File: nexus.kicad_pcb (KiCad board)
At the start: 2 copper layers, 101.5 x 126.2 mm, 112 parts, among them J1 PIN6-9_Breakout, J10 Screw_Terminal_01x02, J11 24V_Lockout_Key_Switch, J12 XT60-M, J13 PT_1, J14 PT_4, J15 PT_2, J16 PT_5, J17 PT_3, J18 PT_6, J19 4-Pin Load Cell, J2 PIN10-13_Breakout, J20 5-Pin Load Cell, J21 Ignitor Screw Terminal, J3 Valve_1_PWR, J4 Valve_4_PWR, J5 Valve_2_PWR, J6 Valve_5_PWR, J7 Valve_3_PWR, J8 Valve_6_PWR, J9 Screw_Terminal_01x04, K1 G5LE-1, K2 G5LE-1, Q1 BSS138, Q2 BSS138, Q3 BSS138, Q4 BSS138, Q5 BSS138, Q6 BSS138, Q7 BSS138, Q8 BSS138, U1 ESP32-S3, U2 ADS112C04, U3 ADS112C04, U4 ADS112C04, U5 ADS112C04, U6 XC6206P332MR, U7 TPS5430DDA, U8 TPS5430DDA

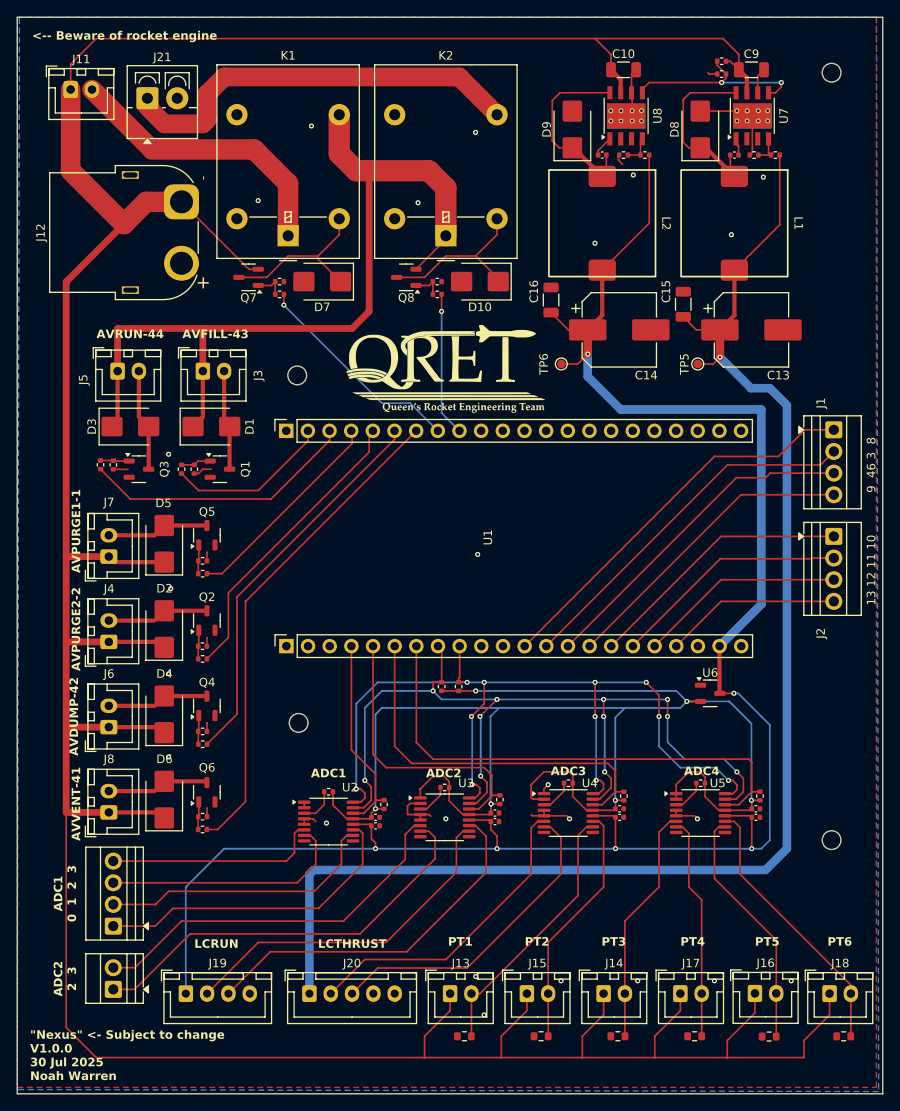
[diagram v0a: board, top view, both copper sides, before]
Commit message: PANDA Rebrand
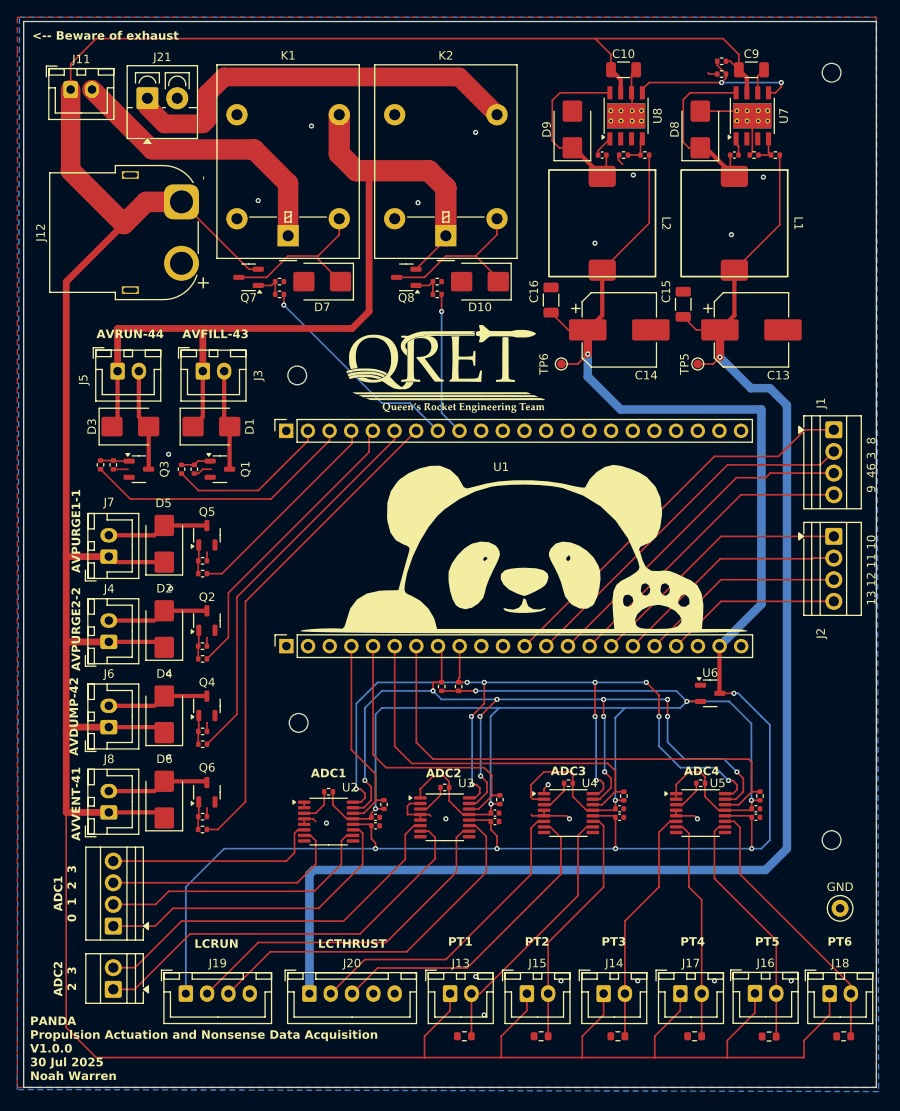
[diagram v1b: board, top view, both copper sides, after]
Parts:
- added G***: LOGO, LOGO, F.Cu at (169.0, 85.7)
- added GND: TestPoint_Loop_D2.50mm_Drill1.0mm, TestPoint:TestPoint_Loop_D2.50mm_Drill1.0mm, F.Cu at (206.0, 128.8)
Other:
- board size 101.5 x 126.2 mm -> 100 x 125 mm
- board text added: "<-- Beware of exhaust"
- board text added: "PANDA Propulsion Actuation and Nonsense Data Acquisition V1.0.0 30 Jul 2025 Noah Warren"
- board text removed: "<-- Beware of rocket engine"
- board text removed: "{dblquote}Nexus{dblquote} <- Subject to change V1.0.0 30 Jul 2025 Noah Warren"
